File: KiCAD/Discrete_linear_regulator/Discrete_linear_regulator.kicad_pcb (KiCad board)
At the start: 4 copper layers, 50 x 36 mm, 40 parts, among them J1 Conn_01x06, Q1 PZT2222AT3G, Q10 BC857, Q11 BC857, Q2 BC857, Q3 BC857, Q4 PZT2222AT3G, Q5 PZT2907AT3G, Q8 PZT2907AT3G, U1 LM4562

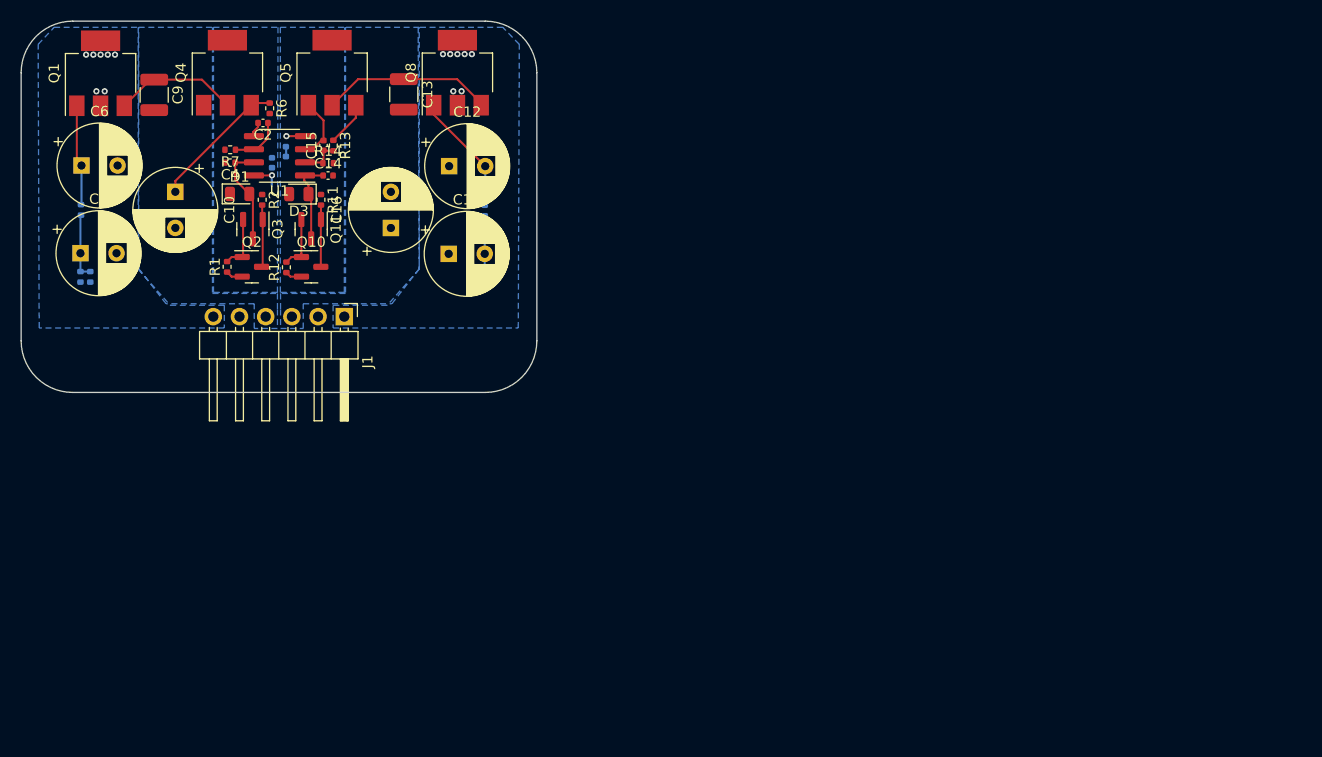
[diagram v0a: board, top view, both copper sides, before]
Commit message: update linear regulators
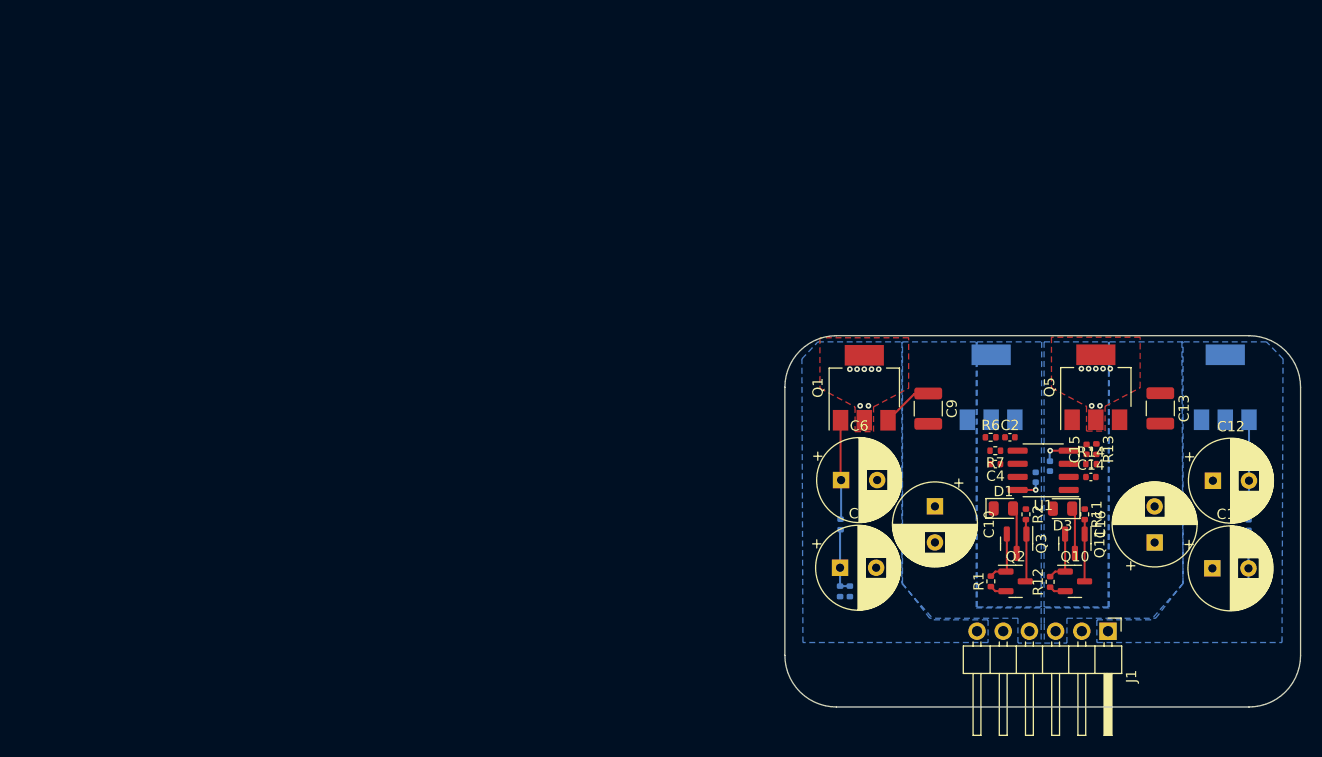
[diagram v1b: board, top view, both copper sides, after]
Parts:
- Q4, Q8: moved to B.Cu
- moved C9 81.0 mm to (137.9, 87.6)
- moved Q8 80.5 mm to (166.8, 85.5)
- moved C3 80.1 mm to (149.8, 93.1)
- moved C1 80.1 mm to (148.4, 94.2)
- moved C11 80.1 mm to (165.5, 103.1)
- moved C12 80.1 mm to (165.5, 94.6)
- moved C16 80.1 mm to (159.9, 100.5)
- moved D3 80.1 mm to (151.0, 97.3)
- moved J1 80.1 mm to (155.4, 109.1)
- moved Q1 80.1 mm to (131.8, 85.5)
- moved Q3 80.1 mm to (146.5, 100.7)
- moved Q4 80.1 mm to (144.1, 85.5)
- moved R1 80.1 mm to (144.0, 104.3)
- moved R10 80.1 mm to (169.0, 98.9)
- moved R11 80.1 mm to (153.1, 97.8)
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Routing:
- net V-: track 21.2 -> 4.54 mm, vias 1 -> 8
- net +12V: track 13.3 -> 0.00 mm
- net V+: track 16.3 -> 8.22 mm
- net Net-(C15-Pad2): track 6.55 -> 0.16 mm
- net Net-(U1B-+): track 5.16 -> 0.00 mm
- net Net-(D1-A): track 9.88 -> 4.89 mm
- net -12V: track 4.30 -> 0.00 mm
- net Net-(D3-K): track 8.40 -> 4.59 mm
- net Net-(U1A-+): track 4.46 -> 1.08 mm
- net Net-(C12-Pad2): track 11.8 -> 9.72 mm
- net Net-(C2-Pad2): track 1.49 -> 0.00 mm
- net -15V: vias 8 -> 0
- net +15V: vias 6 -> 7
- added copper zone on F.Cu, net +15V
- added copper zone on F.Cu, net V-
